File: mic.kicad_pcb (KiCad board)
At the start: 2 copper layers, 50 x 50 mm, 50 parts, among them J1 AudioPlug3, J2 USB_C_Receptacle_USB2.0_16P, SW1 SW_Push, U1 TS5A3159ADBVR, U2 INA826AID, U3 PCM2902CDBR, U4 TLV70033_SOT23-5, U5 USBLC6-2SC6, U6 74LVC1G74DP, Y1 12MHz

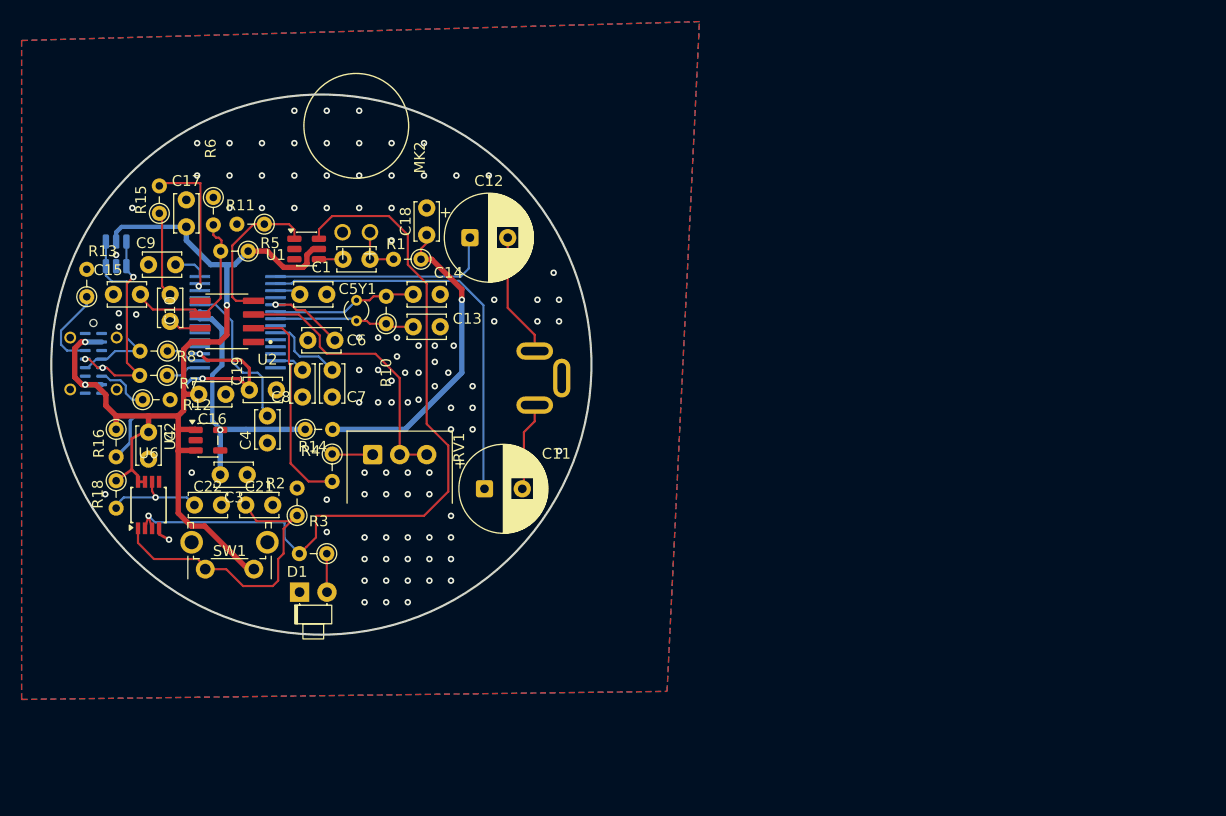
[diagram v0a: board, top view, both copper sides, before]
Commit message: smd version, took only few hours
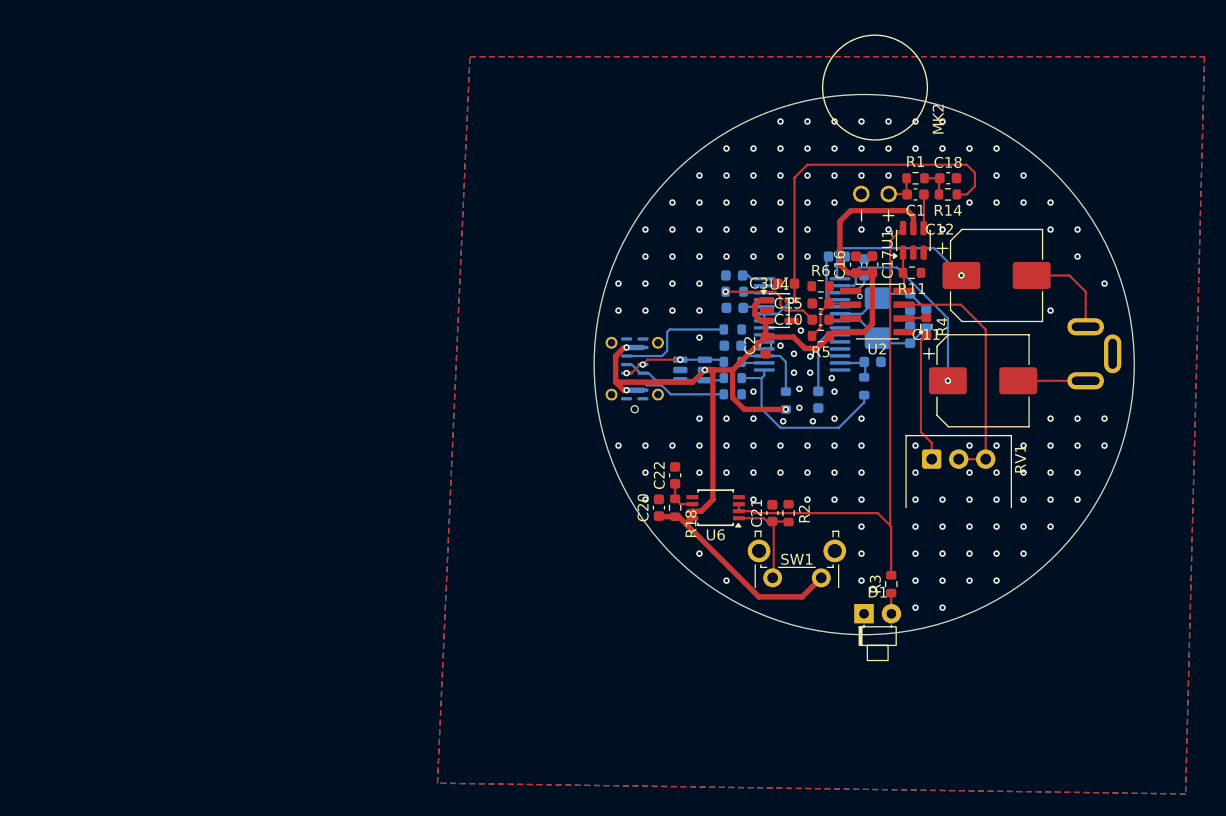
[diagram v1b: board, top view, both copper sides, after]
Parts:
- added C20: 100n, Capacitor_SMD:C_0603_1608Metric, F.Cu at (131.2, 113.2)
- added R9: 1k5R, Resistor_SMD:R_0603_1608Metric, B.Cu at (150.2, 102.0)
- C1, C10, C15, C16, C17, C18, C2, C21, C22, C3: footprint Capacitor_THT:C_Disc_D3.4mm_W2.1mm_P2.50mm -> Capacitor_SMD:C_0603_1608Metric
- C11, C12: footprint Capacitor_THT:CP_Radial_D8.0mm_P3.50mm -> Capacitor_SMD:CP_Elec_8x10
- C13, C14, C19, C4, C5, C6, C7, C8, C9: footprint Capacitor_THT:C_Disc_D3.4mm_W2.1mm_P2.50mm -> Capacitor_SMD:C_0603_1608Metric; moved to B.Cu
- J2: footprint Connector_USB:USB_C_Receptacle_G-Switch_GT-USB-7051x -> mic:USB_C_Receptacle_G-Switch_GT-USB-7051x_NoA8
- MK2: footprint AOM-5024L-HD-F-R:MIC_AOM-5024L-HD-F-R -> mic:MIC_AOM-5024L-HD-F-R
- R1, R11, R14, R18, R2, R3, R4, R5, R6: footprint Resistor_THT:R_Axial_DIN0204_L3.6mm_D1.6mm_P2.54mm_Vertical -> Resistor_SMD:R_0603_1608Metric
- R10, R12, R13, R15, R16, R7, R8: footprint Resistor_THT:R_Axial_DIN0204_L3.6mm_D1.6mm_P2.54mm_Vertical -> Resistor_SMD:R_0603_1608Metric; moved to B.Cu
- U2: footprint INA826AID:SOIC127P599X175-8N -> mic:SOIC127P599X175-8N
- U3: footprint PCM2902C:SOP65P780X200-28N -> mic:SOP65P780X200-28N
- Y1: footprint Crystal:Crystal_C26-LF_D2.1mm_L6.5mm_Vertical -> Crystal:Crystal_SMD_5032-2Pin_5.0x3.2mm; moved to B.Cu
- moved C15 65.5 mm to (146.2, 94.3)
- moved C17 63.8 mm to (151.0, 90.7)
- moved R14 63.4 mm to (158.0, 84.2), turned to 180 degrees
- moved R16 62.1 mm to (143.0, 103.3), turned to 90 degrees
- moved R13 60.5 mm to (138.1, 102.8), turned to 0 degrees
- moved C10 60.3 mm to (146.2, 95.8), turned to 0 degrees
- moved U2 60.2 mm to (151.5, 95.1)
- moved R11 60.1 mm to (154.7, 91.5), turned to 0 degrees
- moved C16 59.6 mm to (149.5, 90.8), turned to -90 degrees
- moved C2 58.1 mm to (141.1, 98.2)
- moved R6 56.8 mm to (146.2, 92.8), turned to 0 degrees
- moved R4 56.2 mm to (156.0, 96.5), turned to 90 degrees
- moved U1 56.2 mm to (154.8, 88.5), turned to 90 degrees
- moved C3 55.3 mm to (143.0, 92.5), turned to 180 degrees
- moved R12 55.0 mm to (138.1, 96.8)
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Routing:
- net Net-(C18-Pad1): track 29.2 -> 2.96 mm, vias 1 -> 0
- net Net-(U6-D): track 71.7 -> 47.9 mm, vias 1 -> 0
- net Net-(U6-C): track 28.8 -> 10.0 mm
- net Net-(U3-VOUTL): track 37.3 -> 19.1 mm, vias 0 -> 1
- net Net-(U2-RG_2): track 20.0 -> 2.08 mm
- net Net-(U3-VBUS): track 25.5 -> 7.52 mm, vias 2 -> 0
- net Net-(U3-D+): track 3.32 -> 17.4 mm
- net Net-(U3-VCCCI): track 14.5 -> 1.99 mm
- net Net-(U3-VINL): track 14.4 -> 2.62 mm, vias 1 -> 0
- net Net-(U2-+IN): track 14.5 -> 3.60 mm
- net +3.3V: track 25.1 -> 35.9 mm
- net +5V: track 93.9 -> 103.2 mm, vias 3 -> 4
- net /USB_DP: track 18.7 -> 9.73 mm, vias 3 -> 0
- net Net-(U2-REF): track 16.2 -> 7.32 mm
- net /USB_DM: track 18.0 -> 9.60 mm, vias 0 -> 3
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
